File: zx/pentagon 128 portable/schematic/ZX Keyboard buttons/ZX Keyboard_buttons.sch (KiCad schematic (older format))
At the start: 51 parts, among them IC1 SN74LS245DW, IC2 SN74LS27N, IC3 SN74LS245DW, J1 Conn_01x03, J2 Conn_01x14, J3 Conn_01x02

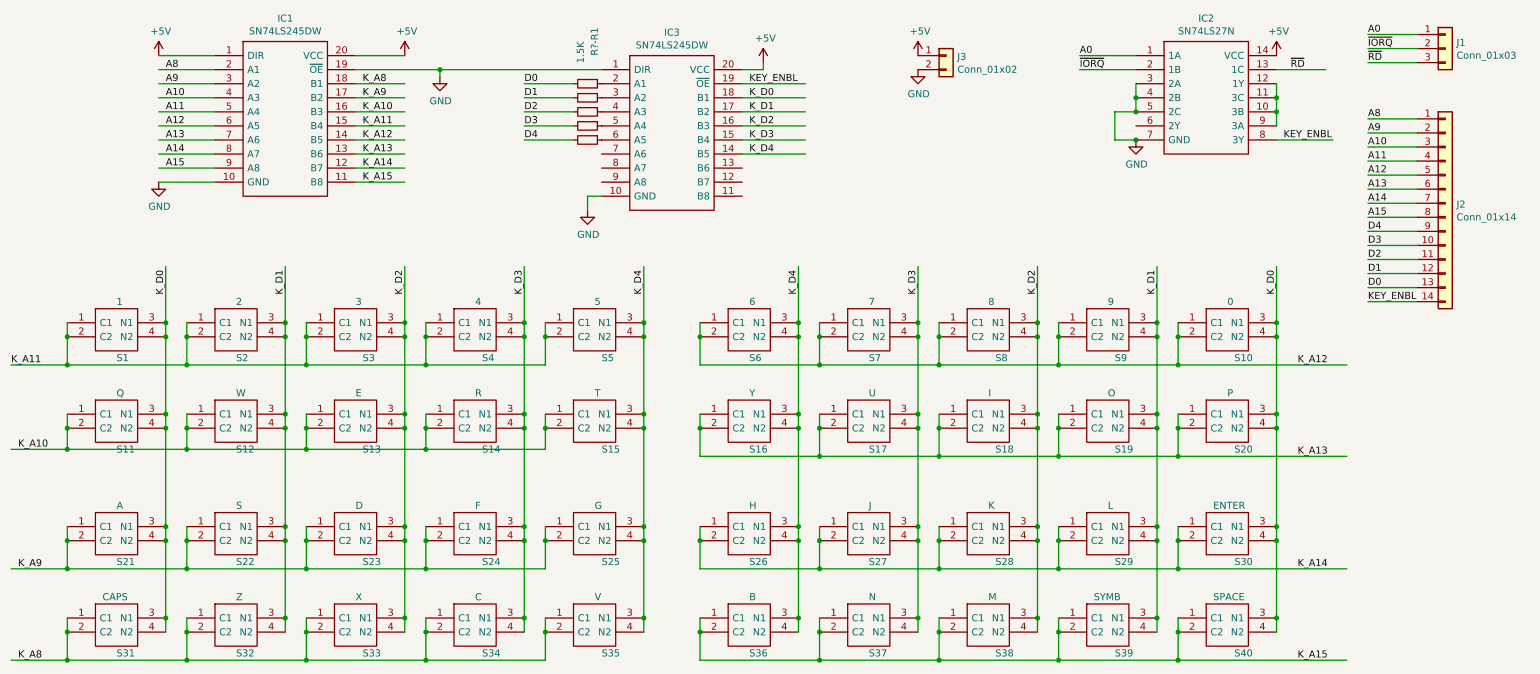
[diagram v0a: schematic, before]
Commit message: fixed keyboard
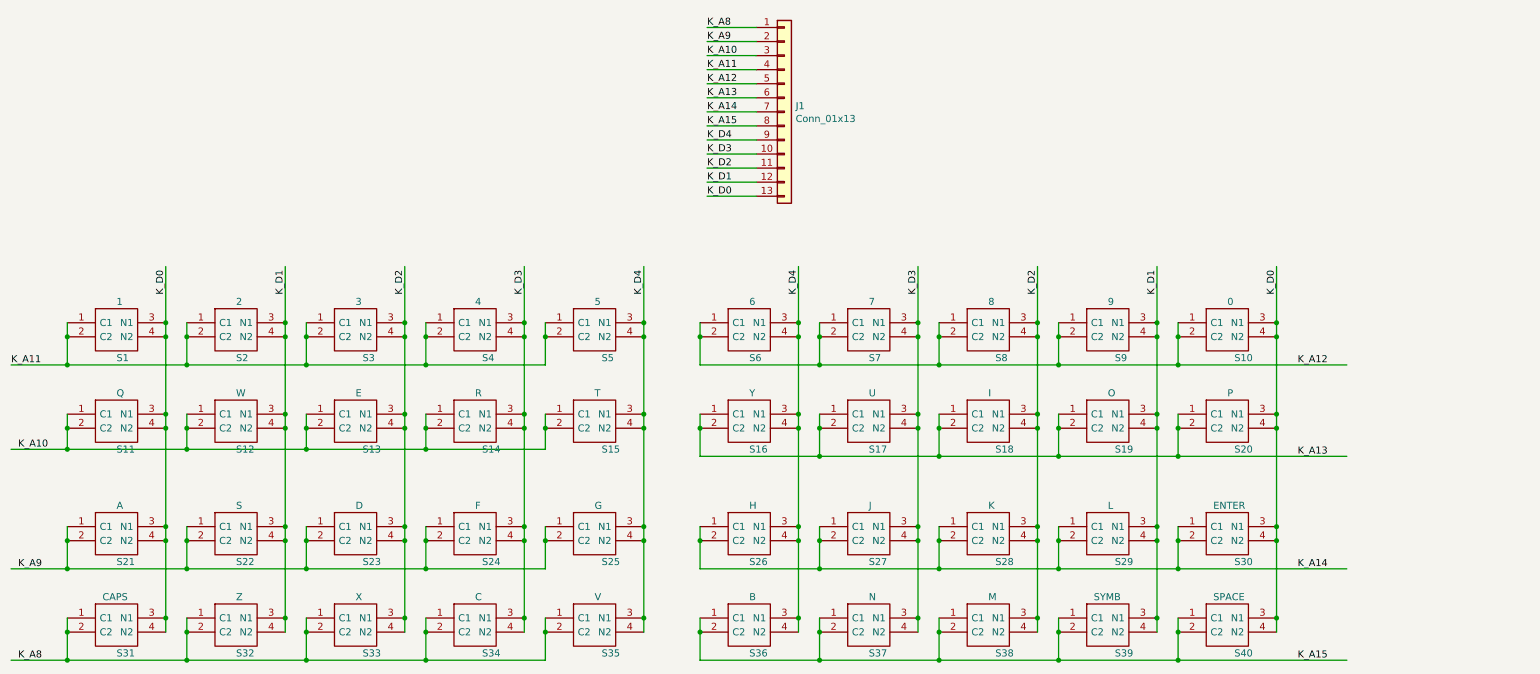
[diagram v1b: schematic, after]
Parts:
- removed IC1, IC3: SN74LS245DW, SamacSys_Parts:SOIC127P1030X265-20N, symbol SamacSys_Parts:SN74LS245DW
- removed IC2: SN74LS27N, SamacSys_Parts:DIP794W53P254L1930H508Q14N, symbol SamacSys_Parts:SN74LS27N
- removed J1: Conn_01x03, Connector_PinHeader_2.54mm:PinHeader_1x03_P2.54mm_Vertical, symbol Connector_Generic:Conn_01x03
- removed J2: Conn_01x14, Connector_PinHeader_2.54mm:PinHeader_1x14_P2.54mm_Vertical, symbol Connector_Generic:Conn_01x14
- removed J3: Conn_01x02, Connector_PinHeader_2.54mm:PinHeader_1x02_P2.54mm_Vertical, symbol Connector_Generic:Conn_01x02
- removed R1, R2, R3, R4, R?-R1: 1.5K, Resistor_SMD:R_0402_1005Metric, symbol Device:R_Small
- added J1: Conn_01x13, Connector_PinHeader_2.54mm:PinHeader_1x13_P2.54mm_Vertical, symbol Connector_Generic:Conn_01x13
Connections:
- net labels removed: +5V, A0, A10, A11, A12, A13, A14, A15, A8, A9, D0, D1, D2, D3, D4, GND, KEY_ENBL, ~IORQ, ~RD
- wire segments 266 -> 213
